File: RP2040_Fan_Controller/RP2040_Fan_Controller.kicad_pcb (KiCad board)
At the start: 2 copper layers, 68.5 x 70 mm, 30 parts

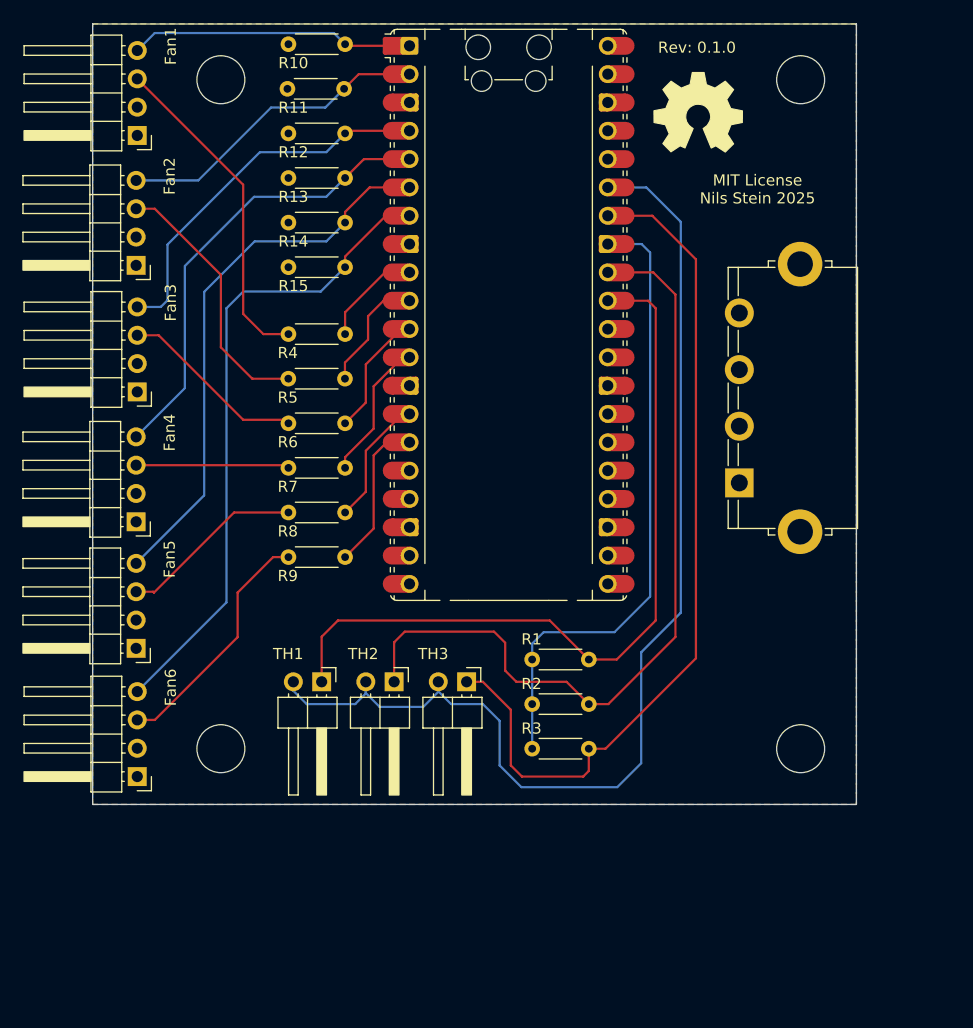
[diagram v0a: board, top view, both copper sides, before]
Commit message: PCB-Rev 0.3.0
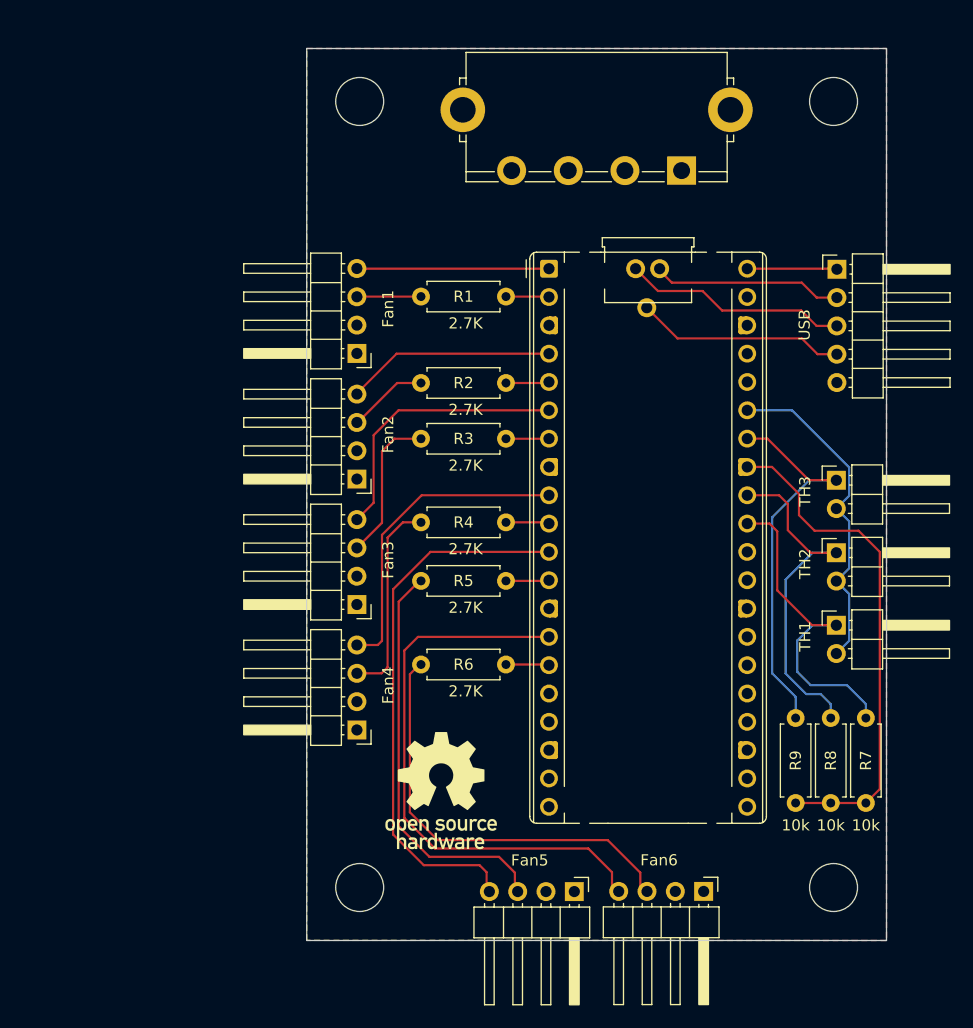
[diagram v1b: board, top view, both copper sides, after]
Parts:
- removed R10: 10K, Resistor_THT:R_Axial_DIN0204_L3.6mm_D1.6mm_P5.08mm_Horizontal
- removed R11, R12, R13, R14, R15: 10k, Resistor_THT:R_Axial_DIN0204_L3.6mm_D1.6mm_P5.08mm_Horizontal
- added ?: , , F.Cu at (181.7, 69.8)
- added ?: , , F.Cu at (179.5, 69.8)
- added ?: , , F.Cu at (180.5, 73.2)
- added G***: LOGO, Library:LOGO, F.Cu at (162.0, 115.1)
- added J1: USB, Connector_PinHeader_2.54mm:PinHeader_1x05_P2.54mm_Horizontal, F.Cu at (197.6, 69.8)
- A1: footprint Module:RaspberryPi_Pico_Common_Unspecified -> Module:RaspberryPi_Pico_Common_THT
- R1: renamed from R4; footprint Resistor_THT:R_Axial_DIN0204_L3.6mm_D1.6mm_P5.08mm_Horizontal -> Resistor_THT:R_Axial_DIN0207_L6.3mm_D2.5mm_P7.62mm_Horizontal
- R2: renamed from R5; footprint Resistor_THT:R_Axial_DIN0204_L3.6mm_D1.6mm_P5.08mm_Horizontal -> Resistor_THT:R_Axial_DIN0207_L6.3mm_D2.5mm_P7.62mm_Horizontal
- R3: renamed from R6; footprint Resistor_THT:R_Axial_DIN0204_L3.6mm_D1.6mm_P5.08mm_Horizontal -> Resistor_THT:R_Axial_DIN0207_L6.3mm_D2.5mm_P7.62mm_Horizontal
- R4: renamed from R7; footprint Resistor_THT:R_Axial_DIN0204_L3.6mm_D1.6mm_P5.08mm_Horizontal -> Resistor_THT:R_Axial_DIN0207_L6.3mm_D2.5mm_P7.62mm_Horizontal
- R5: renamed from R8; footprint Resistor_THT:R_Axial_DIN0204_L3.6mm_D1.6mm_P5.08mm_Horizontal -> Resistor_THT:R_Axial_DIN0207_L6.3mm_D2.5mm_P7.62mm_Horizontal
- R6: renamed from R9; footprint Resistor_THT:R_Axial_DIN0204_L3.6mm_D1.6mm_P5.08mm_Horizontal -> Resistor_THT:R_Axial_DIN0207_L6.3mm_D2.5mm_P7.62mm_Horizontal
- R7: renamed from R1; footprint Resistor_THT:R_Axial_DIN0204_L3.6mm_D1.6mm_P5.08mm_Horizontal -> Resistor_THT:R_Axial_DIN0207_L6.3mm_D2.5mm_P7.62mm_Horizontal
- R8: renamed from R2; footprint Resistor_THT:R_Axial_DIN0204_L3.6mm_D1.6mm_P5.08mm_Horizontal -> Resistor_THT:R_Axial_DIN0207_L6.3mm_D2.5mm_P7.62mm_Horizontal
- R9: renamed from R3; footprint Resistor_THT:R_Axial_DIN0204_L3.6mm_D1.6mm_P5.08mm_Horizontal -> Resistor_THT:R_Axial_DIN0207_L6.3mm_D2.5mm_P7.62mm_Horizontal
- moved REF** 73.5 mm to (154.8, 125.2)
- moved REF** 59.4 mm to (154.8, 54.8)
- moved Fan6 51.8 mm to (185.6, 125.6), turned to -90 degrees
- moved TH1 46.4 mm to (197.5, 101.7), turned to 0 degrees
- moved Fan5 44.9 mm to (174.0, 125.6), turned to -90 degrees
- moved TH2 41.3 mm to (197.5, 95.2), turned to 0 degrees
- moved TH3 37.8 mm to (197.5, 88.7), turned to 0 degrees
- moved R7 32.6 mm to (200.2, 117.7), turned to 90 degrees
- moved REF** 28.5 mm to (183.6, 61.0), turned to 180 degrees
- moved R8 28.2 mm to (197.0, 117.7), turned to 90 degrees
- moved Fan1 27.8 mm to (154.5, 77.3)
- moved Fan2 27.6 mm to (154.5, 88.6)
- moved Fan3 27.4 mm to (154.5, 99.9)
- moved Fan4 27.2 mm to (154.5, 111.1)
- moved R9 24.1 mm to (193.8, 117.7), turned to 90 degrees
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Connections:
- net Net-(A1-ADC_VREF) renamed ADC_VREF
- net Net-(A1-AGND) renamed ADC_GND
- net Net-(A1-GPIO0) renamed PWM_FAN1
- net Net-(A1-GPIO11) renamed RPM_FAN6
- net Net-(A1-GPIO26_ADC0) renamed ADC_0
- net Net-(A1-GPIO27_ADC1) renamed ADC_1
- net Net-(A1-GPIO28_ADC2) renamed ADC_2
- A1 pad 10: Net-(A1-GPIO7) -> RPM_FAN4
- A1 pad 11: Net-(A1-GPIO8) -> PWM_FAN5
- A1 pad 12: Net-(A1-GPIO9) -> RPM_FAN5
- A1 pad 14: Net-(A1-GPIO10) -> PWM_FAN6
- A1 pad 2: Net-(A1-GPIO1) -> RPM_FAN1
- A1 pad 4: Net-(A1-GPIO2) -> PWM_FAN2
- A1 pad 40: unconnected-(A1-VBUS-Pad40) -> VBUS
- A1 pad 5: Net-(A1-GPIO3) -> RPM_FAN2
- A1 pad 6: Net-(A1-GPIO4) -> PWM_FAN3
- A1 pad 7: Net-(A1-GPIO5) -> RPM_FAN3
- A1 pad 9: Net-(A1-GPIO6) -> PWM_FAN4
- Fan2 pad 4: Net-(A1-GPIO1) -> PWM_FAN2
- Fan3 pad 4: Net-(A1-GPIO2) -> PWM_FAN3
- Fan4 pad 4: Net-(A1-GPIO3) -> PWM_FAN4
- Fan5 pad 4: Net-(A1-GPIO4) -> PWM_FAN5
- Fan6 pad 4: Net-(A1-GPIO5) -> PWM_FAN6
- R1 pad 2: Net-(A1-GPIO6) -> RPM_FAN1
- R2 pad 2: Net-(A1-GPIO7) -> RPM_FAN2
- R3 pad 2: Net-(A1-GPIO8) -> RPM_FAN3
- R4 pad 2: Net-(A1-GPIO9) -> RPM_FAN4
- R5 pad 2: Net-(A1-GPIO10) -> RPM_FAN5
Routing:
- net ADC_VREF: track 102.4 -> 30.3 mm
- net Net-(A1-GPIO5): track 58.1 -> 0.00 mm
- net PWM_FAN6: track 0.00 -> 50.9 mm
- net Net-(A1-GPIO4): track 49.7 -> 0.00 mm
- net PWM_FAN5: track 0.00 -> 49.0 mm
- net ADC_2: track 77.1 -> 35.8 mm
- net Net-(A1-GPIO3): track 41.3 -> 0.00 mm
- net ADC_1: track 72.6 -> 32.2 mm
- net ADC_0: track 69.3 -> 30.6 mm
- net Net-(A1-GPIO2): track 34.2 -> 0.00 mm
- net Net-(A1-GPIO1): track 29.1 -> 0.00 mm
- net PWM_FAN4: track 0.00 -> 29.0 mm
- net PWM_FAN3: track 0.00 -> 25.5 mm
- net Net-(Fan1-Tacho): track 29.8 -> 5.70 mm
- net USB_DP: track 0.00 -> 20.2 mm
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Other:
- board size 68.5 x 70 mm -> 52 x 80 mm
- board text added: "Rev: 1.0.0 MIT License Nils Stein 2025"
- board text removed: "MIT License Nils Stein 2025"
- board text removed: "Rev: 0.1.0"
